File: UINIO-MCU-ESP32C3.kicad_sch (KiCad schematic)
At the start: 1 part

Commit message: update
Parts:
- added AE?: Antenna, symbol Device:Antenna
- added C? (x7): 0.1uF, symbol Device:C
- added C? (x2): 0.1uF, Capacitor_SMD:C_0603_1608Metric, symbol Device:C
- added C?: 1uF, Capacitor_SMD:C_0603_1608Metric, symbol Device:C
- added C? (x2): 15pF, symbol Device:C
- added C? (x2): 1uF, Capacitor_SMD:C_0402_1005Metric, symbol Uinio:CAP_0402
- added C? (x2): 1uF, symbol Device:C
- added C?: 10nF, symbol Device:C
- added D? (x2): BLUE LED, LED_SMD:LED_0603_1608Metric, symbol Device:LED
- added D?: Green LED, LED_SMD:LED_0603_1608Metric, symbol Device:LED
- added F?: Polyfuse, Fuse:Fuse_1206_3216Metric, symbol Device:Polyfuse
- added J?: 外接串行下载接口, symbol Connector:Conn_01x04_Male
- added L?: L, symbol Device:L
- added R? (x3): 10K, symbol Device:R
- added R?: 0R, symbol Device:R
- added R? (x3): 2K, Resistor_SMD:R_0603_1608Metric, symbol Device:R
- added SW?: 下载按键, Uinio:KEY-SMD_4P-L4.2-W3.4-P2.15-LS4.7, symbol Uinio:Key_YTS_A016S_1
- added SW?: 复位按键, Uinio:KEY-SMD_4P-L4.2-W3.4-P2.15-LS4.7, symbol Uinio:Key_YTS_A016S_1
- added U?: W25Q128JVSSIQ, kicad_lceda:SOIC-8_L5.3-W5.3-P1.27-LS8.0-BL, symbol Uinio:W25Q128JVSSIQ
- added U?: CH343P, kicad_lceda:TQFN-16_L3.0-W3.0-P0.50-BL-EP1.7, symbol Uinio:CH343P
- added U?: ME6211C33M5G-N, Uinio:SOT-23-5_L3.0-W1.7-P0.95-LS2.8-BR, symbol Uinio:ME6211
- added USB?: USB_Type_C_16Pin, Uinio:USB-C-SMD_TYPEC-304J-BCP16, symbol Uinio:USB_Type_C_16Pin
- added VT? (x2): S8050, Uinio:SOT-23-3_L2.9-W1.6-P1.90-LS2.9-BL, symbol Uinio:S8050
- added Y?: Crystal_GND24, symbol Device:Crystal_GND24
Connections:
- net at U?.1 (LNA_IN): now also C?.1, L?.2
- net GPIO5/ADC2/SCL: now reaches U?.10 (MTDI)
- net SPIHD: now reaches U?.11 (VDD3P3_RTC)
- net SPIHD: now also U?.17 (VDD3P3_CPU), U?.2 (VDD3P3), U?.3 (VDD3P3), U?.31 (VDDA), U?.32 (VDDA), C?.1, C?.1, C?.1, C?.1, C?.1, C?.1, C?.1, C?.2, R?.2, U?.3 (WP#(IO2)), U?.5 (Vout), U?.7 (HOLD#/RESET#/(IO3)), U?.8 (VCC)
- net GPIO6: now reaches U?.12 (MTCK)
- net GPIO7: now reaches U?.13 (MTDO)
- net GPIO8/PWM: now reaches U?.14 (GPIO8)
- net GPIO9/BOOT: now reaches U?.15 (GPIO9)
- net GPIO9/BOOT: now also R?.1, SW?.3, SW?.4, VT?.3 (C)
- net GPIO10: now reaches U?.16 (GPIO10)
- net VDD_SPI/GPIO11: now reaches U?.18 (VDD_SPI)
- net VDD_SPI/GPIO11: now also C?.1
- net SPIHD/GPIO12: now reaches U?.19 (SPIHD)
- net SPIWP/GPIO13: now reaches U?.20 (SPIWP)
- net SPICS0: now reaches U?.21 (SPICS0)
- net SPICS0: now also U?.1 (CS#)
- net SPICLK: now reaches U?.22 (SPICLK)
- net SPICLK: now also U?.6 (CLK)
- net SPID: now reaches U?.23 (SPID)
- net SPID: now also U?.5 (DI(IO0))
- net SPIQ: now reaches U?.24 (SPIQ)
- net SPIQ: now also U?.2 (DO(IO1))
- net GPIO18/USB_D-: now reaches U?.25 (GPIO18)
- net GPIO19/USB_D+: now reaches U?.26 (GPIO19)
- net U0RXD: now reaches U?.27 (U0RXD)
- net U0RXD: now also J?.3 (Pin_3)
- net U0TXD: now reaches U?.28 (U0TXD)
- net U0TXD: now also J?.2 (Pin_2)
- net at U?.29 (XTAL_N): now also C?.2, Y?.3
- net at U?.30 (XTAL_P): now also R?.2
- net GND: now reaches U?.33 (EP)
- net GND: now also C?.1, C?.1, C?.1, C?.1, C?.1, C?.1, C?.2, C?.2, C?.2, C?.2, C?.2, C?.2, C?.2, C?.2, C?.2, C?.2, C?.2, D?.1 (K), SW?.1, SW?.1, SW?.2, SW?.2, U?.17 (EP), U?.2 (GND), U?.2 (Vss), U?.4 (GND), USB?.13 (GND), USB?.14 (GND), USB?.15 (GND), USB?.16 (GND), USB?.A1B12 (GND), USB?.B1A12 (GND), Y?.2, Y?.4
- net GPIO0/U1TXD: now reaches U?.4 (XTAL_32K_P)
- net GPIO1/U1RXD: now reaches U?.5 (XTAL_32K_N)
- net GPIO2: now reaches U?.6 (GPIO2)
- net CHIP_EN: now reaches U?.7 (CHIP_EN)
- net CHIP_EN: now also SW?.3, SW?.4, VT?.3 (C)
- net GPIO3: now reaches U?.8 (GPIO3)
- net GPIO4/ADC1/SDA: now reaches U?.9 (MTMS)
- new net: R?.2, VT?.1 (B) (x2)
- new net: C?.2, R?.1, Y?.1
- new net: AE?.1 (A), C?.1, L?.1
- new net: D?.1 (K), R?.2 (x2)
- new net: D?.2 (A), R?.1
- new net: F?.1, USB?.A4B9 (VBUS), USB?.B4A9 (VBUS)
- new net CH343_ACT#: U?.10 (ACT#)
- new net CH343_CTS: U?.15 (CTS)
- new net CH343_DCD: U?.11 (DCD)
- new net CH343_DSR: U?.14 (DSR)
- new net CH343_DTR: U?.12 (DTRTNOW)
- new net CH343_RI: U?.16 (RI)
- new net CH343_RTS: U?.13 (RTS)
- new net CH343_RXD: R?.1, U?.5 (RXD)
- new net CH343_TXD: R?.1, U?.4 (TXD)
- new net CH343_USB_Data_N: U?.8 (UD-), USB?.A7 (DN1), USB?.B7 (DN2)
- new net CH343_USB_Data_P: U?.7 (UD+), USB?.A6 (DP1), USB?.B6 (DP2)
- new net CH343_VDD_3.3V: C?.2, U?.6 (V3)
- new net CH343_VDD_5V: C?.2, F?.2, R?.2, U?.3 (VDD5), U?.9 (VBUS)
- new net CH343_VIO: C?.1, D?.2 (A), D?.2 (A), U?.1 (VIO)
- new net DTR: J?.1 (Pin_1), R?.1, VT?.2 (E)
- new net RTS: J?.4 (Pin_4), R?.1, VT?.2 (E)
- new net VDD_5V: C?.2, U?.1 (Vin), U?.3 (CE)
- no-connect marks 0 -> 5
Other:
- note added: "ME6211C33M5G-N 供电电路"
- moved on the sheet: U?

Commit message: update
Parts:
- removed D? (x2): BLUE LED, LED_SMD:LED_0603_1608Metric, symbol Device:LED
- removed R? (x2): 2K, Resistor_SMD:R_0603_1608Metric, symbol Device:R
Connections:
- net CH343_DTR is gone; now on net DTR: U?.12 (DTRTNOW)
- net CH343_RTS is gone; now on net RTS: U?.13 (RTS)
- net CH343_VDD_3.3V is gone; now on net SPIHD: C?.2, U?.6 (V3)
- net CH343_VIO is gone; now on net SPIHD: C?.1, U?.1 (VIO)
- net CH343_VDD_5V: no longer C?.2, U?.3 (VDD5), U?.9 (VBUS)
- net VDD_5V: now also C?.2, U?.3 (VDD5), U?.9 (VBUS)
- net CH343_ACT#: no longer names the net of U?.10 (ACT#)
- net CH343_CTS: no longer names the net of U?.15 (CTS)
- net CH343_DCD: no longer names the net of U?.11 (DCD)
- net CH343_DSR: no longer names the net of U?.14 (DSR)
- net CH343_RI: no longer names the net of U?.16 (RI)
- net CH343_RXD renamed RXD
- net CH343_TXD renamed TXD
- net CH343_USB_Data_N renamed USB_Data-
- net USB_Data-: no longer USB?.B7 (DN2)
- net CH343_USB_Data_P renamed USB_Data+
- net USB_Data+: no longer USB?.B6 (DP2)
- new net USB_Data_N: USB?.B7 (DN2)
- new net USB_Data_P: USB?.B6 (DP2)
- no-connect marks 5 -> 10
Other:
- moved on the sheet: AE?, C?, D?, F?, J?, L?, R?, SW?, U?, USB?, VT?, Y?

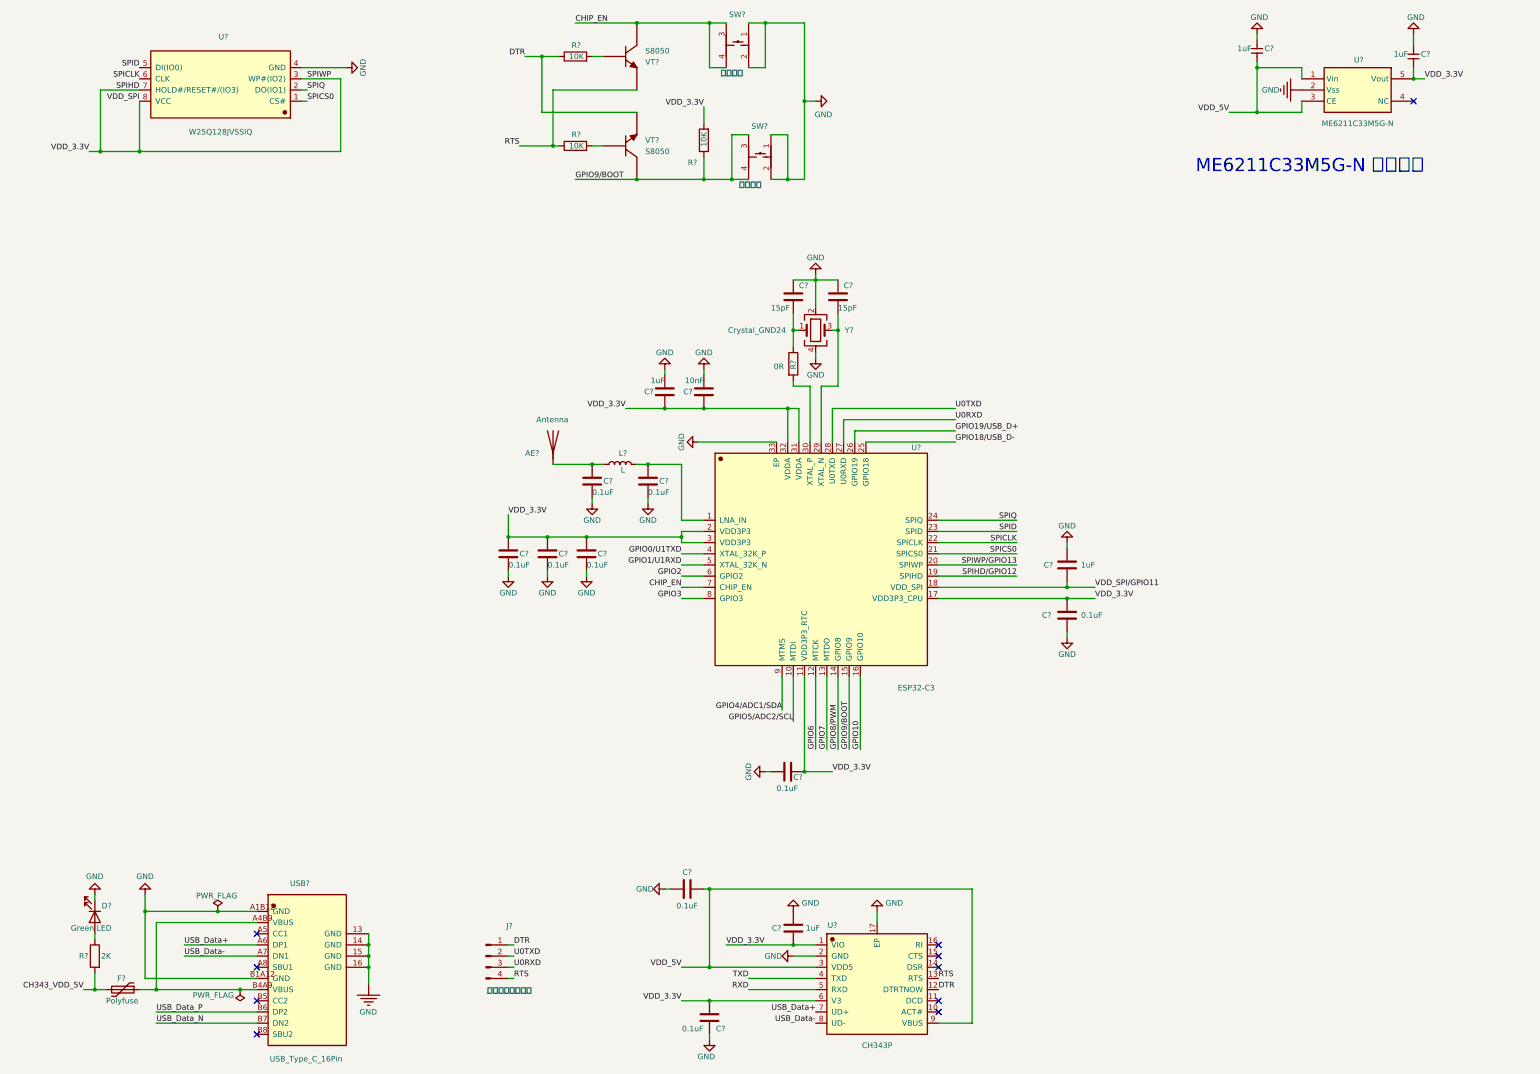
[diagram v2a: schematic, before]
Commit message: update
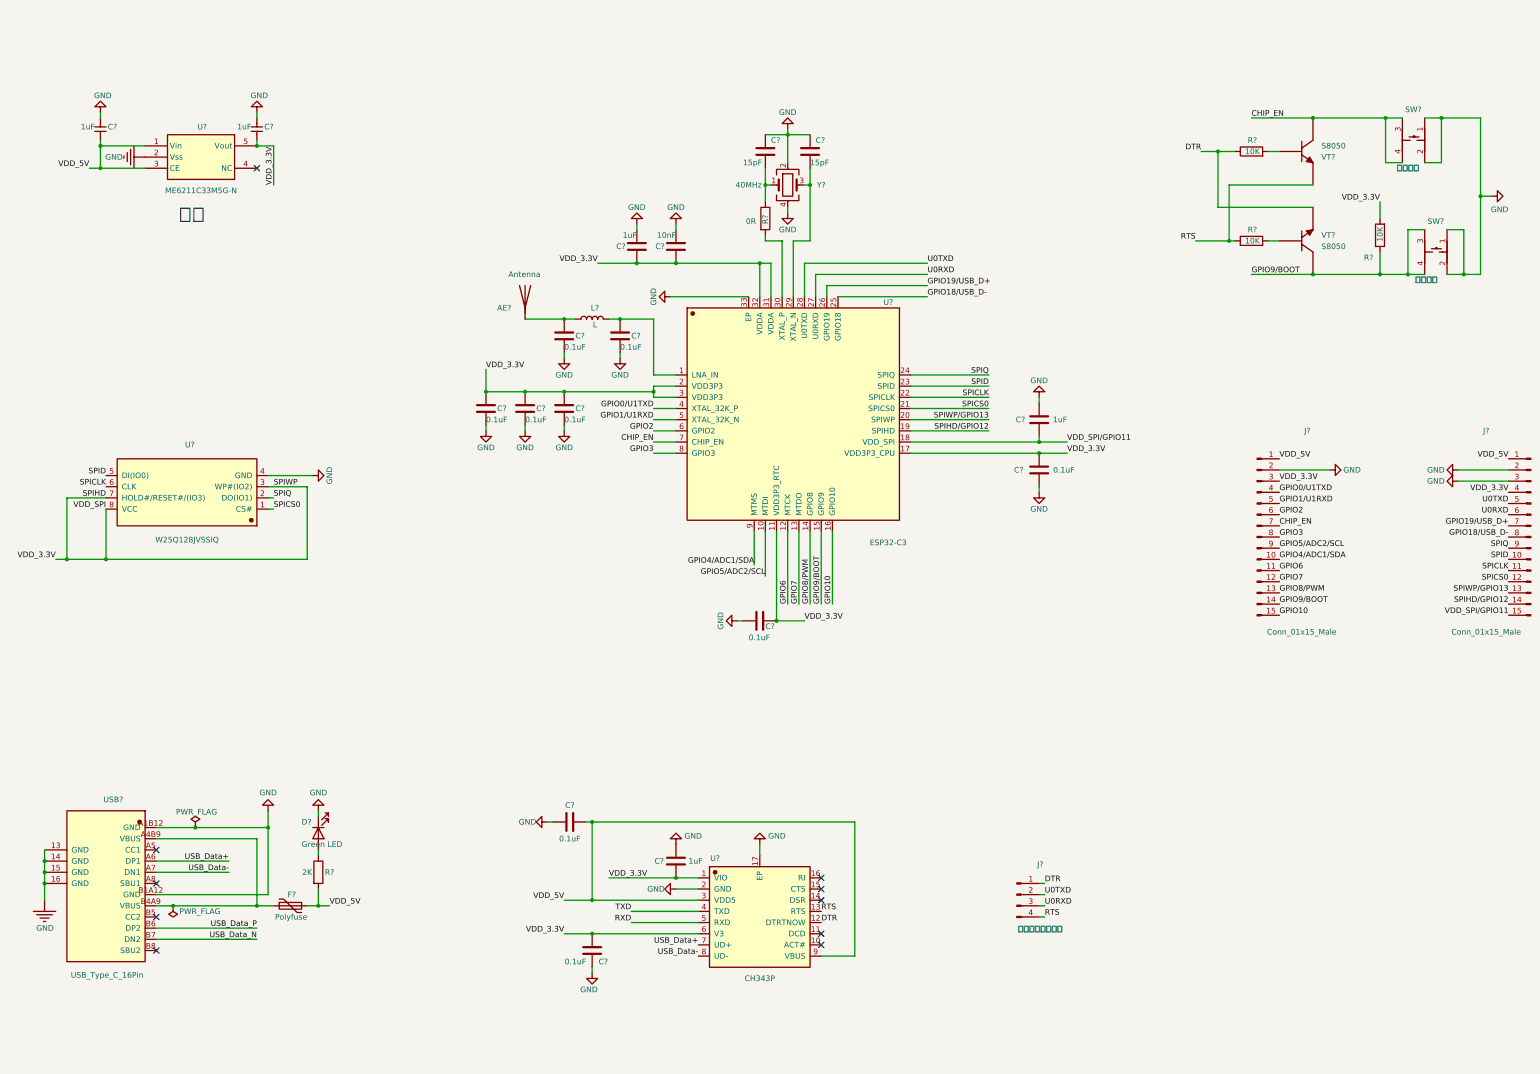
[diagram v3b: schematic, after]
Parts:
- added J? (x2): Conn_01x15_Male, symbol Connector:Conn_01x15_Male
- Y?: value Crystal_GND24 -> 40MHz
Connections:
- net CH343_VDD_5V is gone; now on net VDD_5V: F?.2, R?.2
- net CHIP_EN: now also J?.7 (Pin_7)
- net GND: now also J?.2 (Pin_2), J?.2 (Pin_2), J?.3 (Pin_3)
- net GPIO0/U1TXD: now also J?.4 (Pin_4)
- net GPIO10: now also J?.15 (Pin_15)
- net GPIO18/USB_D-: now also J?.8 (Pin_8)
- net GPIO19/USB_D+: now also J?.7 (Pin_7)
- net GPIO1/U1RXD: now also J?.5 (Pin_5)
- net GPIO2: now also J?.6 (Pin_6)
- net GPIO3: now also J?.8 (Pin_8)
- net GPIO4/ADC1/SDA: now also J?.10 (Pin_10)
- net GPIO5/ADC2/SCL: now also J?.9 (Pin_9)
- net GPIO6: now also J?.11 (Pin_11)
- net GPIO7: now also J?.12 (Pin_12)
- net GPIO8/PWM: now also J?.13 (Pin_13)
- net GPIO9/BOOT: now also J?.14 (Pin_14)
- net SPICLK: now also J?.11 (Pin_11)
- net SPICS0: now also J?.12 (Pin_12)
- net SPID: now also J?.10 (Pin_10)
- net SPIHD: now also J?.3 (Pin_3), J?.4 (Pin_4)
- net SPIHD/GPIO12: now also J?.14 (Pin_14)
- net SPIQ: now also J?.9 (Pin_9)
- net SPIWP/GPIO13: now also J?.13 (Pin_13)
- net U0RXD: now also J?.6 (Pin_6)
- net U0TXD: now also J?.5 (Pin_5)
- net VDD_5V: now also J?.1 (Pin_1), J?.1 (Pin_1)
- net VDD_SPI/GPIO11: now also J?.15 (Pin_15)
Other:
- note added: "电源"
- note removed: "ME6211C33M5G-N 供电电路"
- moved on the sheet: AE?, C?, D?, F?, J?, L?, R?, SW?, U?, USB?, VT?, Y?
